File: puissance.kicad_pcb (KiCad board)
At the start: 4 copper layers, 65 x 43 mm, 37 parts, among them J5 Screw_Terminal_01x10, J8 MEC1-110-02-F-D-A, J9 Screw_Terminal_01x04, K5 G6DN-1A-L DC24, K6 G6DN-1A-L DC24, U11 SIP-4_1779205311, U12 PDRV81545PWPR, U13 ISO7720D, U14 TLV75709PDBV, U8 ISO1212

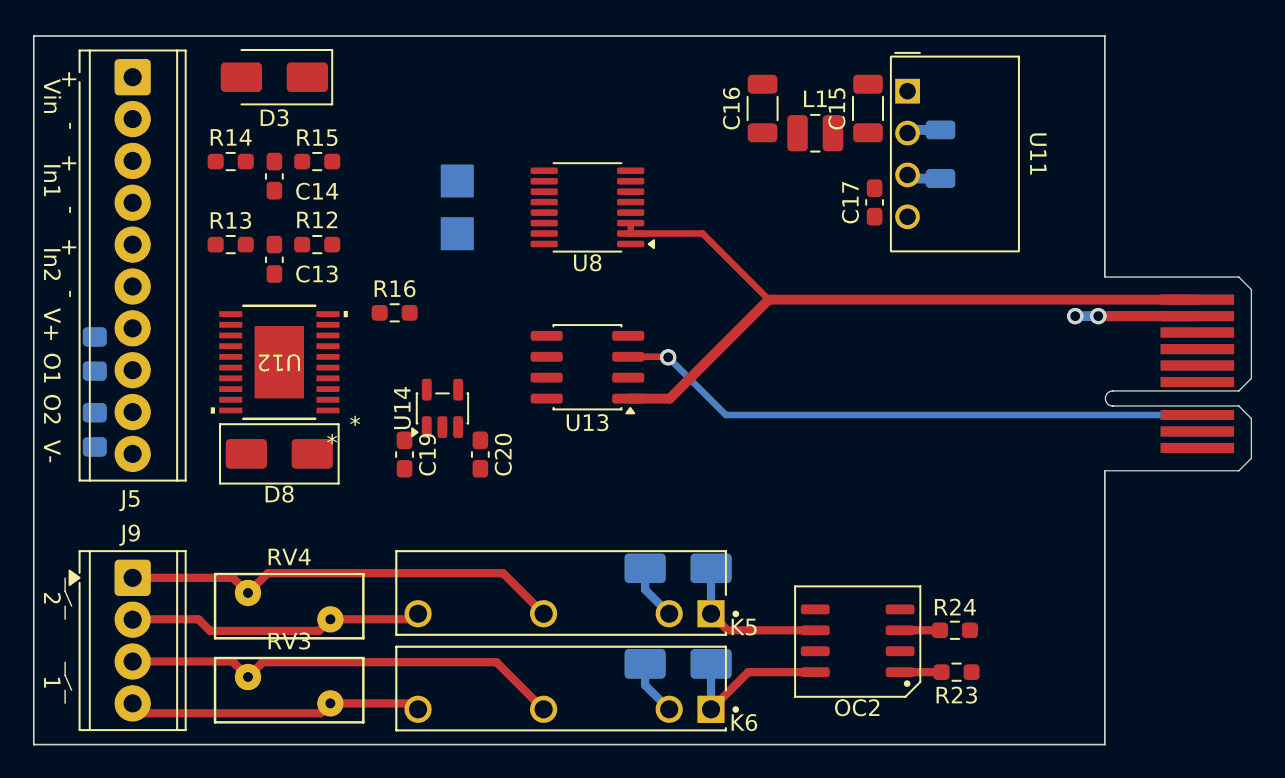
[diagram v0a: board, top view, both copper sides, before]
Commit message: suite et nouvel écran
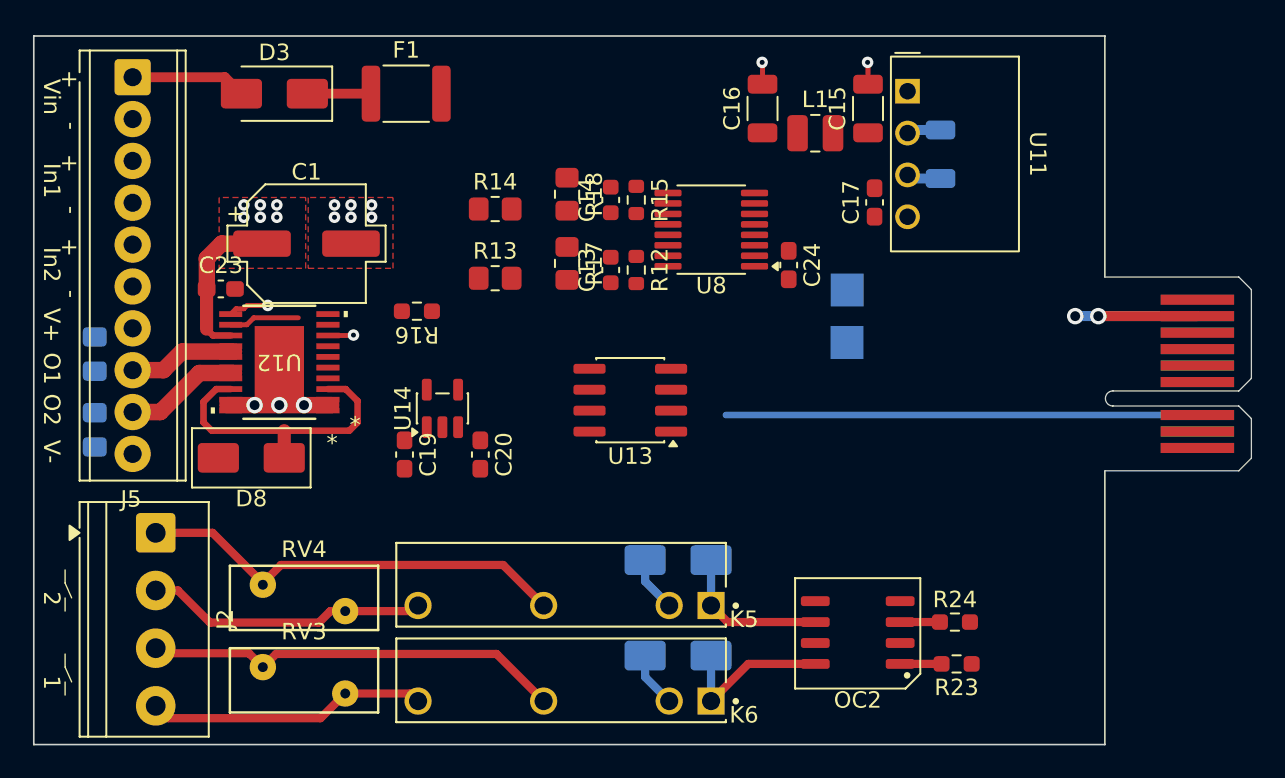
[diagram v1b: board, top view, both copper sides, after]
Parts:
- removed J9: Screw_Terminal_01x04, TerminalBlock_Phoenix:TerminalBlock_Phoenix_MPT-0,5-4-2.54_1x04_P2.54mm_Horizontal
- added C1: 47µ 50V, PCM_Capacitor_SMD_AKL:CP_Elec_6.3x7.7, F.Cu at (116.5, 62.6)
- added C23: 1µ, Capacitor_SMD:C_0603_1608Metric_Pad1.08x0.95mm_HandSolder, F.Cu at (111.3, 65.3)
- added C24: 0.1µ, Capacitor_SMD:C_0603_1608Metric_Pad1.08x0.95mm_HandSolder, F.Cu at (145.8, 63.9)
- added F1: 100mA, Fuse:Fuse_1812_4532Metric, F.Cu at (122.6, 53.5)
- added J2: Screw_Terminal_01x04, TerminalBlock_Phoenix:TerminalBlock_Phoenix_PT-1,5-4-3.5-H_1x04_P3.50mm_Horizontal, F.Cu at (107.4, 80.2)
- added R17: optional, Resistor_SMD:R_0805_2012Metric_Pad1.20x1.40mm_HandSolder, F.Cu at (132.4, 63.8)
- added R18: optional, Resistor_SMD:R_0805_2012Metric_Pad1.20x1.40mm_HandSolder, F.Cu at (132.4, 59.6)
- C13, C14: value 0.1µ -> 10n; footprint Capacitor_SMD:C_0603_1608Metric_Pad1.08x0.95mm_HandSolder -> Capacitor_SMD:C_0603_1608Metric
- R12, R15: value 562 -> 560; footprint Resistor_SMD:R_0603_1608Metric_Pad0.98x0.95mm_HandSolder -> Resistor_SMD:R_0603_1608Metric
- R13, R14: value 2k5 -> 2k4; footprint Resistor_SMD:R_0603_1608Metric_Pad0.98x0.95mm_HandSolder -> Resistor_SMD:R_0805_2012Metric_Pad1.20x1.40mm_HandSolder
- U13: value ISO7720D -> ISO6420FDR
- moved TP1 24.6 mm to (149.4, 65.4)
- moved TP2 24.6 mm to (149.3, 68.6)
- moved C14 20.5 mm to (135.0, 60.0), turned to 90 degrees
- moved C13 20.4 mm to (135.0, 64.2), turned to 90 degrees
- moved R15 19.5 mm to (136.6, 60.0), turned to -90 degrees
- moved R12 19.4 mm to (136.6, 64.2), turned to -90 degrees
- moved R14 16.3 mm to (128.0, 60.5)
- moved R13 16.2 mm to (128.0, 64.7)
- moved U8 7.63 mm to (141.1, 61.8)
- moved U13 3.28 mm to (136.2, 72.1)
- moved D8 1.72 mm to (113.2, 75.6)
- moved R16 1.35 mm to (123.2, 66.7), turned to 180 degrees
- moved RV3 1.08 mm to (118.9, 89.9)
- moved RV4 1.03 mm to (118.9, 84.9)
- moved D3 1.00 mm to (114.6, 53.5)
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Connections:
- net /Input1 renamed /Entrée/Input1
- net /Input2 renamed /Entrée/Input2
- net /Output1 renamed /Sorties/Output2
- net /Output2 renamed /Sorties/Output1
- net Net-(J9-Pin_1) renamed /Sorties/Relais2_COM
- net Net-(J9-Pin_2) renamed /Sorties/Relais2_NO
- net Net-(J9-Pin_3) renamed /Sorties/Relais1_COM
- net Net-(J9-Pin_4) renamed /Sorties/Relais1_NO
- C13 pad 1: Net-(U8-IN1) -> Net-(U8-SENSE1)
- C14 pad 1: Net-(U8-IN2) -> Net-(U8-SENSE2)
- D3 pad 1: +24V -> Net-(D3-K)
- D8 pad 2: /Voutput -> GND2
- J5 pad 10: /Voutput -> unconnected-(J5-Pin_10-Pad10)
- J8 pad 07: /Relay1_MCU -> /Output_6
- J8 pad 08: unconnected-(J8-Pad08) -> /Output_6
- J8 pad 09: /Relay2_MCU -> /Output_5
- J8 pad 10: unconnected-(J8-Pad10) -> /Output_5
- J8 pad 11: /Output1_MCU -> /Output_4
- J8 pad 12: unconnected-(J8-Pad12) -> /Output_4
- J8 pad 15: /Output2_MCU -> /Output_3
- J8 pad 16: unconnected-(J8-Pad16) -> /Output_3
- J8 pad 17: /Input1_MCU -> /Output_2
- J8 pad 18: unconnected-(J8-Pad18) -> /Output_2
- J8 pad 19: /Input2_MCU -> /Output_1
- J8 pad 20: unconnected-(J8-Pad20) -> /Output_1
- R12 pad 1: Net-(U8-SENSE1) -> Net-(U8-IN1)
- R12 pad 2: Net-(U8-IN1) -> Net-(U8-SENSE1)
- R13 pad 2: Net-(U8-IN1) -> Net-(U8-SENSE1)
- R14 pad 2: Net-(U8-IN2) -> Net-(U8-SENSE2)
- R15 pad 1: Net-(U8-SENSE2) -> Net-(U8-IN2)
- R15 pad 2: Net-(U8-IN2) -> Net-(U8-SENSE2)
- R23 pad 1: /Relay1_MCU -> /Output_1
- R24 pad 1: /Relay2_MCU -> /Output_2
- U13 pad 2: /Output1_MCU -> /Sorties/Output1_MCU
- U13 pad 3: /Output2_MCU -> /Sorties/Output2_MCU
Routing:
- net +3V3: track 47.7 -> 0.00 mm
- net /Output2_MCU: track 36.0 -> 0.00 mm, vias 1 -> 0
- net /Output_3: track 0.00 -> 28.6 mm
- net Net-(D8-K): track 0.00 -> 18.0 mm
- net GND2: track 0.00 -> 13.0 mm, vias 0 -> 13
- net +24V: track 6.73 -> 16.4 mm, vias 0 -> 6
- net /Sorties/Output2: track 0.00 -> 7.13 mm
- net Net-(D3-A): track 0.00 -> 7.01 mm
- net /Sorties/Output1: track 0.00 -> 6.84 mm
- net Net-(U12A-ILIM): track 0.00 -> 4.28 mm
- net Net-(D3-K): track 0.00 -> 3.86 mm
- net /Sorties/Relais1_COM: track 26.9 -> 25.5 mm
- net /Sorties/Relais1_NO: track 18.0 -> 17.1 mm
- net /Sorties/Relais2_NO: track 18.0 -> 17.3 mm
- net Net-(U8-SUB2): track 0.00 -> 0.70 mm
- added copper zone on F.Cu, net +24V
- added copper zone on F.Cu, net GND2
